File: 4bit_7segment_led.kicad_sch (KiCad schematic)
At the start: 15 parts, among them U3 74HC595, U4 7segment_4_anode, U5 74HC595

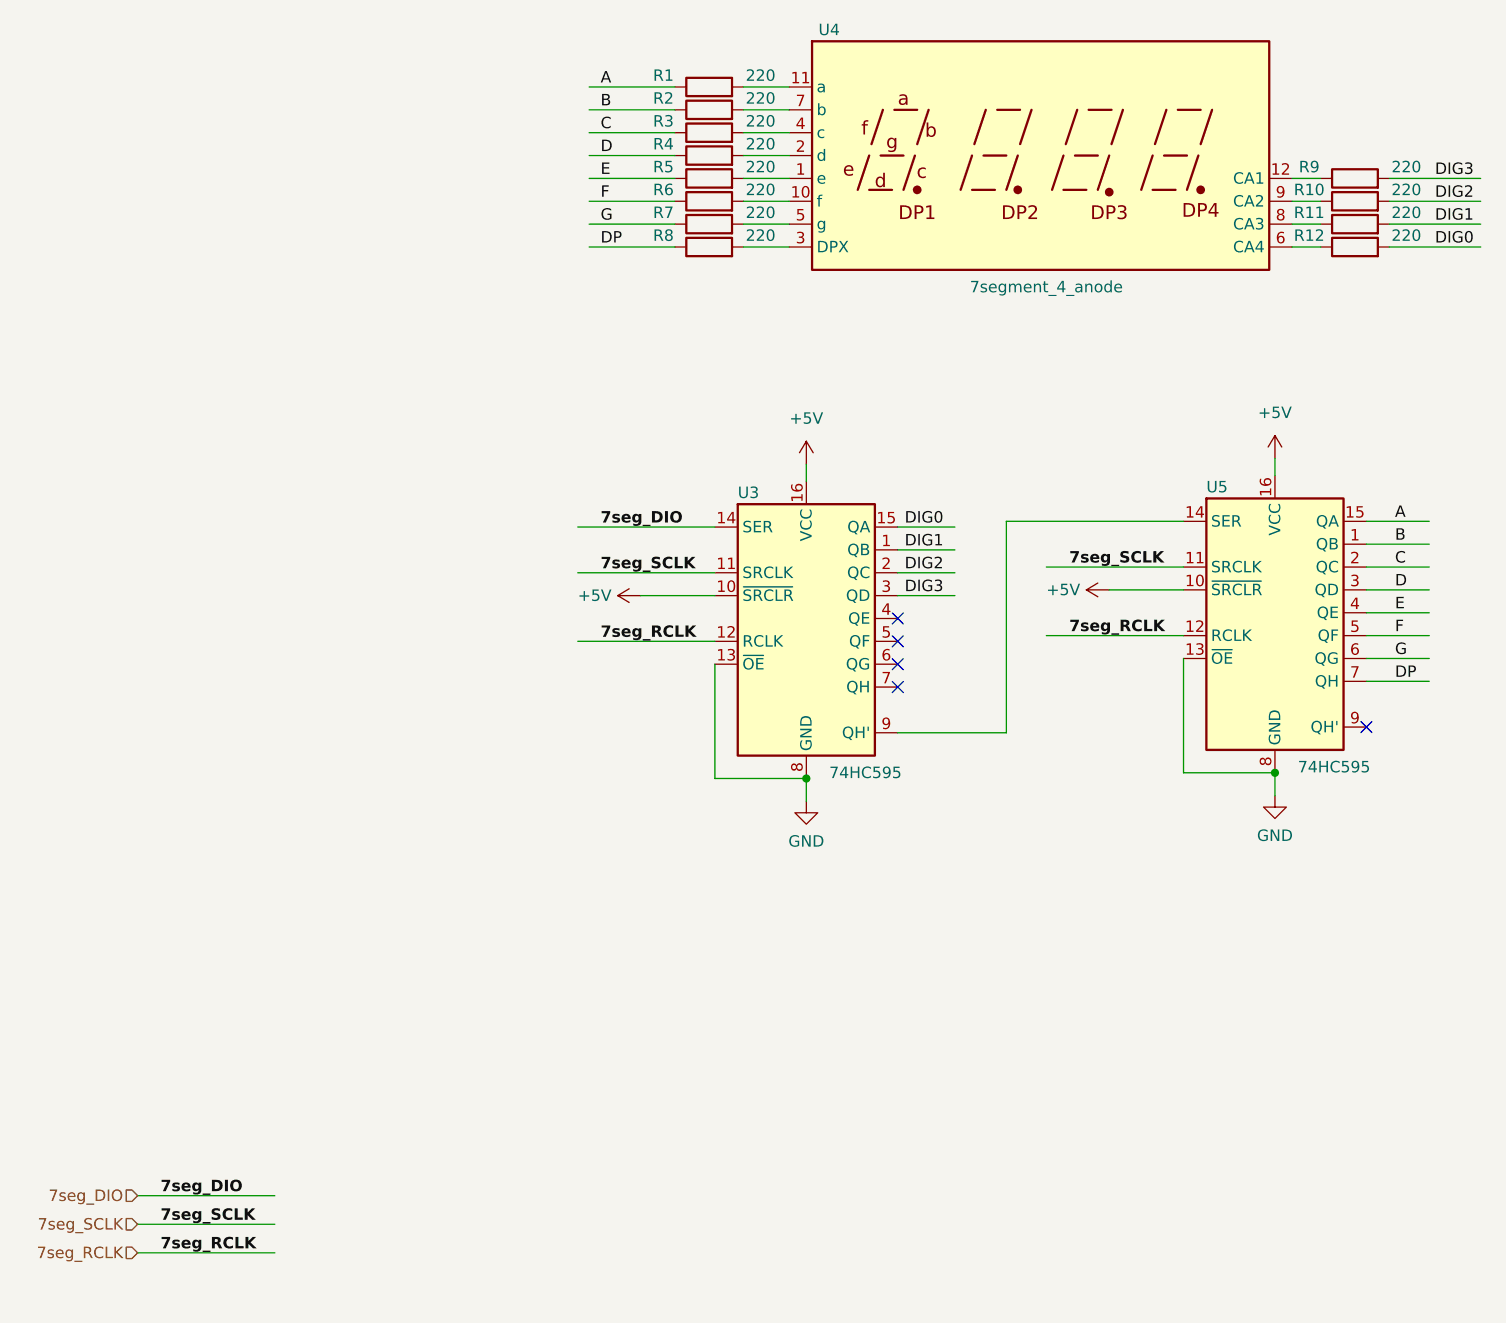
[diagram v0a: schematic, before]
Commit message: modify packet of res
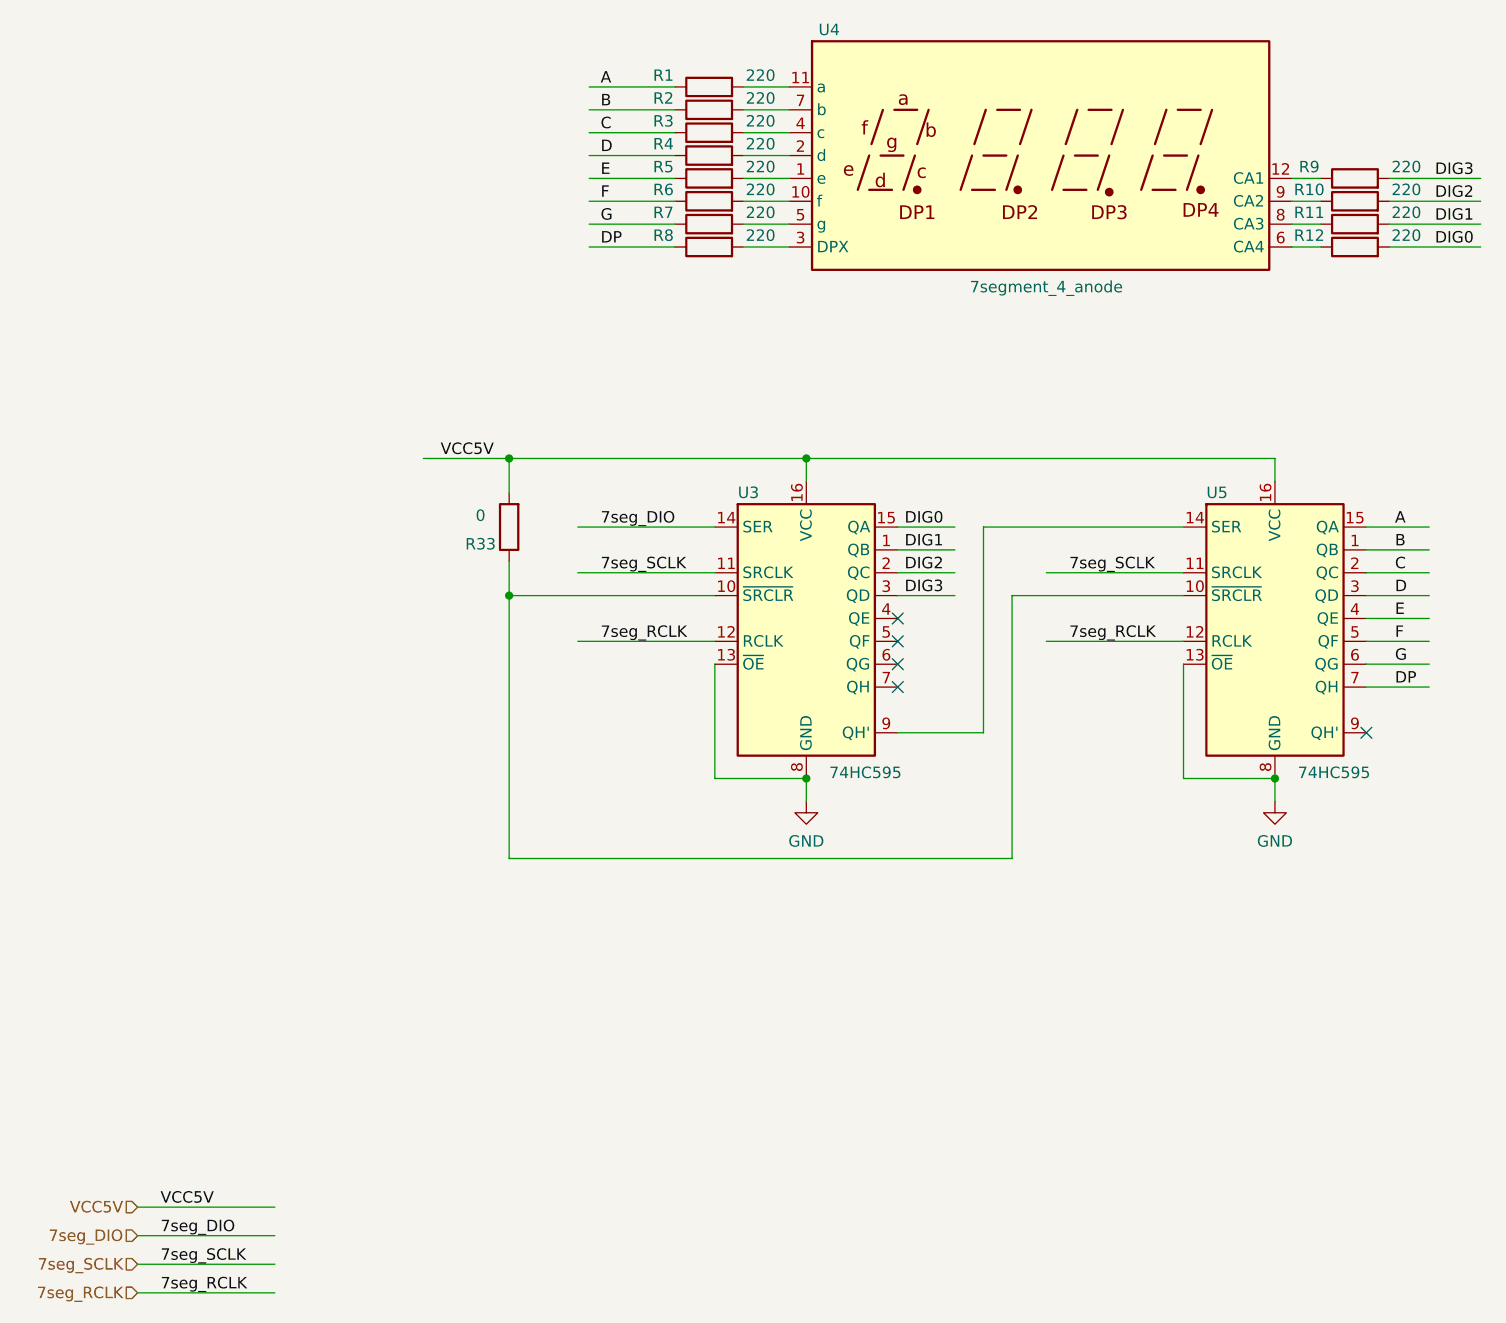
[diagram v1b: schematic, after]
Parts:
- added R33: 0, Resistor_SMD:R_0603_1608Metric, symbol Device:R
- R1, R10, R11, R12, R2, R3, R4, R5, R6, R7, R8, R9: footprint (none) -> Resistor_SMD:R_0603_1608Metric
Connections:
- net +5V: no longer names the net of U3.10 (~{SRCLR}), U5.10 (~{SRCLR})
- net +5V: now also R33.1; no longer U3.16 (VCC), U5.16 (VCC)
- new net VCC5V: R33.2, U3.16 (VCC), U5.16 (VCC)
